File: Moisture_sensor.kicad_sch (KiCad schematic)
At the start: 10 parts, among them J1 Conn_01x02_Socket, U2 TLV2371DBV

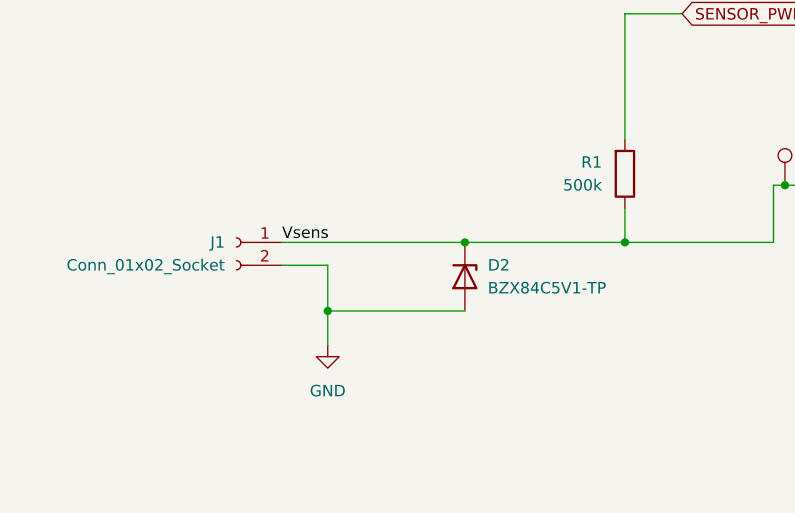
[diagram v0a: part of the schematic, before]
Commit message: laid out pcb
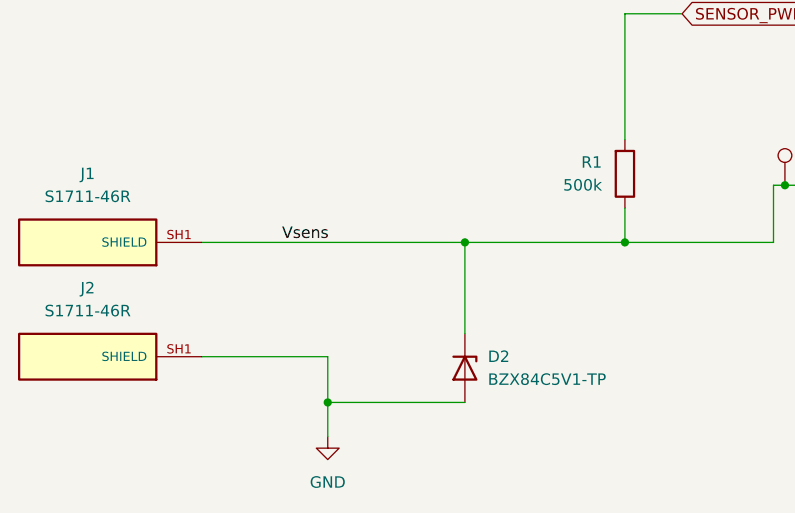
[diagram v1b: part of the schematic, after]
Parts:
- removed J1: Conn_01x02_Socket, Connector_Wire:SolderWire-0.1sqmm_1x02_P3.6mm_D0.4mm_OD1mm_Relief, symbol Connector:Conn_01x02_Socket
- added J1, J2: S1711-46R, Hydro_footprints:HARWIN_S1711-46R, symbol Hydro_symbols:S1711-46R
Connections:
- net GND: now also J2.SH1 (SHIELD)
- net Vsens: now also J1.SH1 (SHIELD)
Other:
- moved on the sheet: D2
